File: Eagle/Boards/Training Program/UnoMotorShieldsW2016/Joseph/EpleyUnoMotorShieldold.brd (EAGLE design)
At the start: 100 x 80 mm, 7 parts, among them J1 ARDUINO_UNO_R3

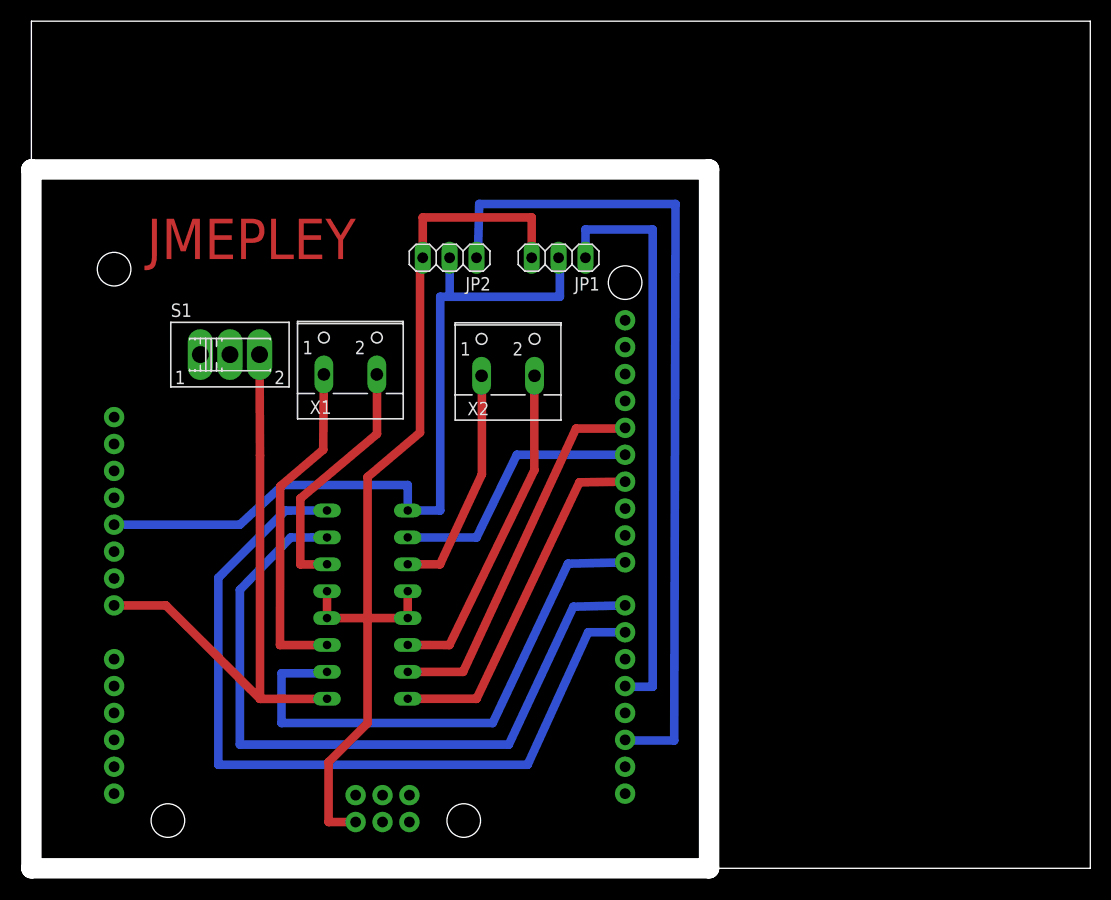
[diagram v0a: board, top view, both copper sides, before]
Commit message: updated Joseph's board
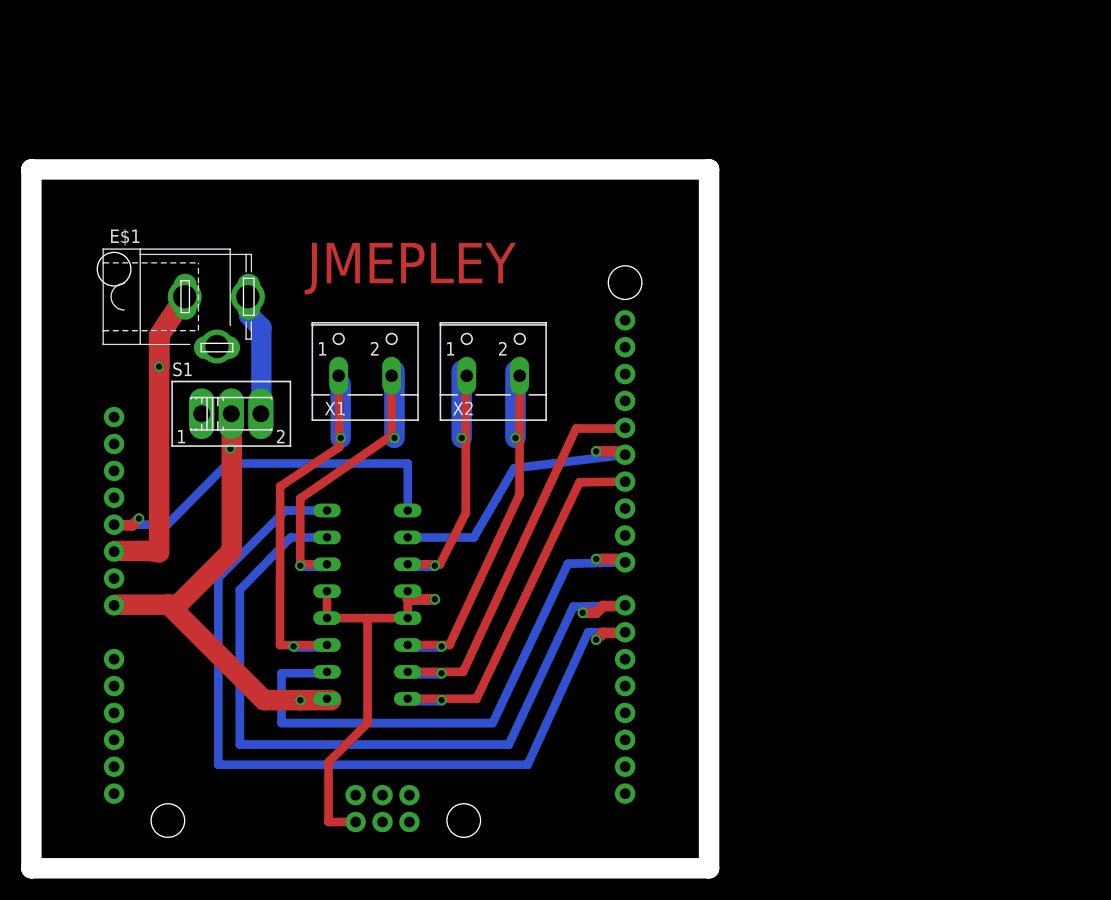
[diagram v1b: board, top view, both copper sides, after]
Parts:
- removed JP1, JP2: (no value), ISCTRainingProgram:1X03
- added E$1: (no value), ISCTRainingProgram:5.5-2.5-BARRELCONNECTOR
- moved S1 5.59 mm to (18.9, 42.9)
- moved X1 1.40 mm to (31.5, 47.8)
- moved X2 1.40 mm to (43.6, 47.8)
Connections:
- removed net N$11: J1.D4, JP1.1
- removed net N$12: J1.5V, JP1.2, JP2.2, U$1.P16
- new net S$1: E$1.P$1
- new net S$4: S1.3
- net GND: no longer JP1.3, JP2.3
- net N$5: now also J1.5V, U$1.P16; no longer J1.D2, JP2.1
- net N$7: no longer S1.3
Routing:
- net N$12: track 73.6 -> 0.00 mm
- net N$11: track 54.9 -> 0.00 mm
- net GND: track 90.4 -> 36.0 mm
- net S$5: track 0.00 -> 47.7 mm, vias 0 -> 1
- net N$5: track 79.1 -> 34.6 mm
- net S$1: track 0.00 -> 36.5 mm, vias 0 -> 1
- net N$7: track 56.3 -> 23.8 mm
- net S$2: track 0.00 -> 11.8 mm
- net S$9: track 0.00 -> 6.35 mm, vias 0 -> 1
- net S$8: track 0.00 -> 6.35 mm, vias 0 -> 1
- net S$7: track 0.00 -> 6.35 mm, vias 0 -> 1
- net S$6: track 0.00 -> 5.08 mm, vias 0 -> 1
- net S$18: track 0.00 -> 5.08 mm, vias 0 -> 1
- net S$21: track 0.00 -> 4.07 mm, vias 0 -> 1
- net S$16: track 0.00 -> 3.18 mm, vias 0 -> 1
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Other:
- board size 100 x 80 mm -> 64 x 66 mm
